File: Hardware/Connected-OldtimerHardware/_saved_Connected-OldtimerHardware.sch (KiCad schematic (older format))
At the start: 20 parts, among them J1 CAN_Bus_Connector, J2 MainConnector, J3 NextionConnector, Q1 2N3906, U1 ParticleElectron, U2 TSR_2-2450, U3 CANTranceiverModule, U4 AdafruitFRAM, U5 AdafruitUltimateGPS, U6 MotionSensor, U7 SFH618A-2

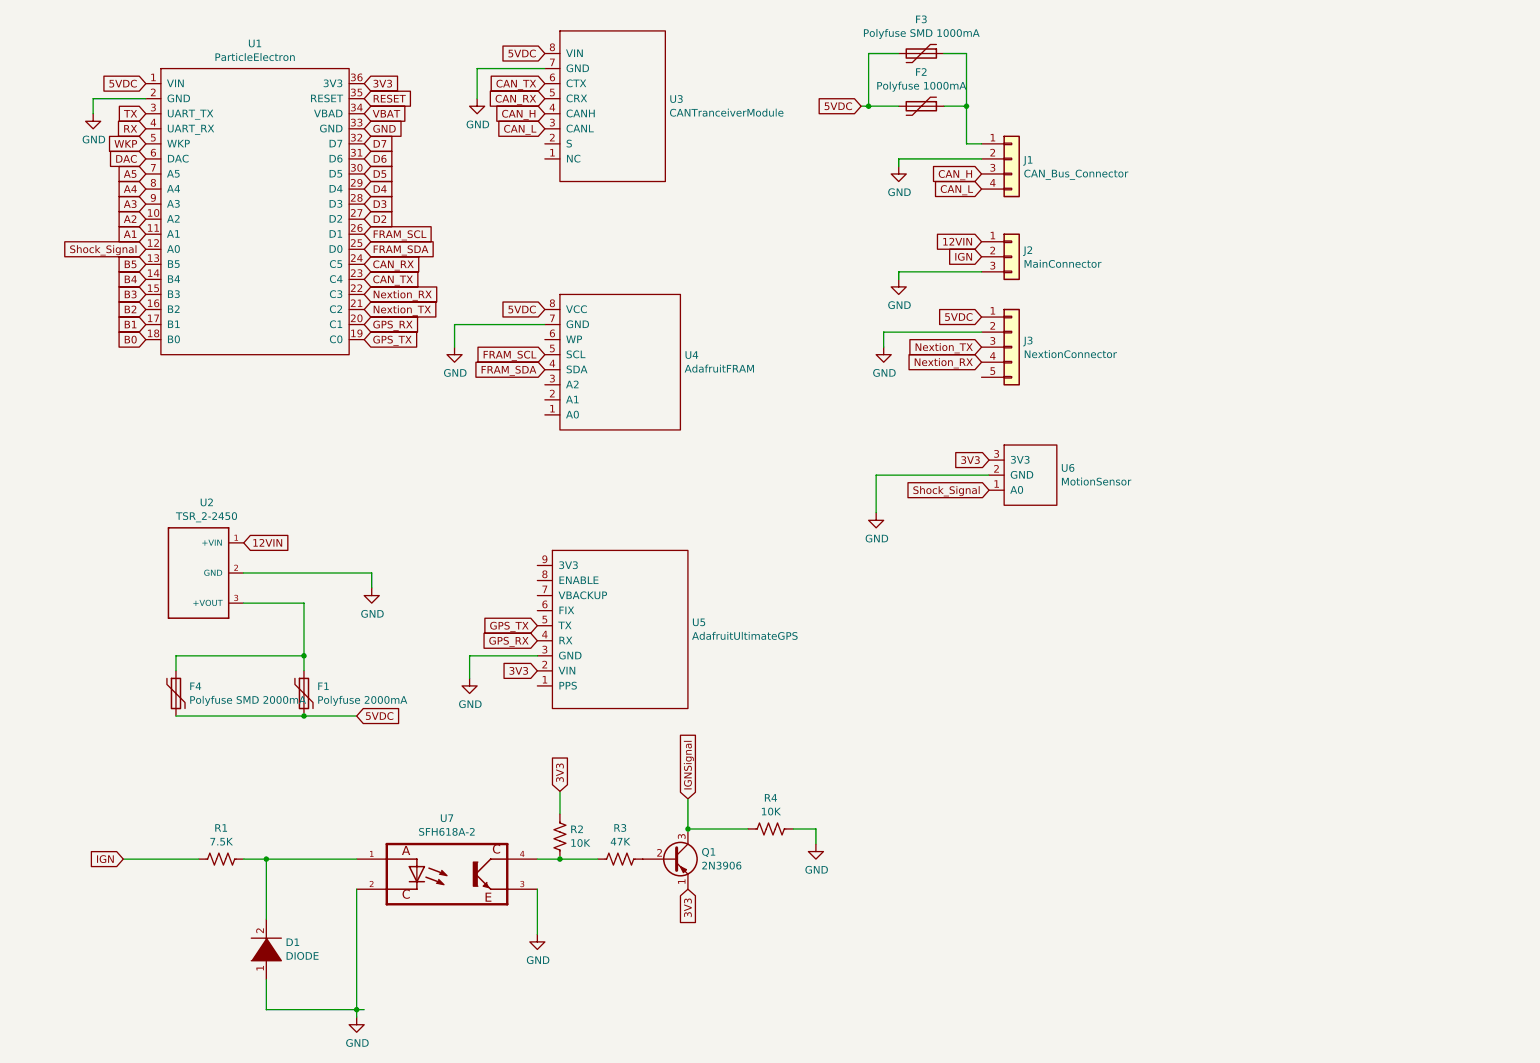
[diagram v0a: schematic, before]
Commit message: layout v1
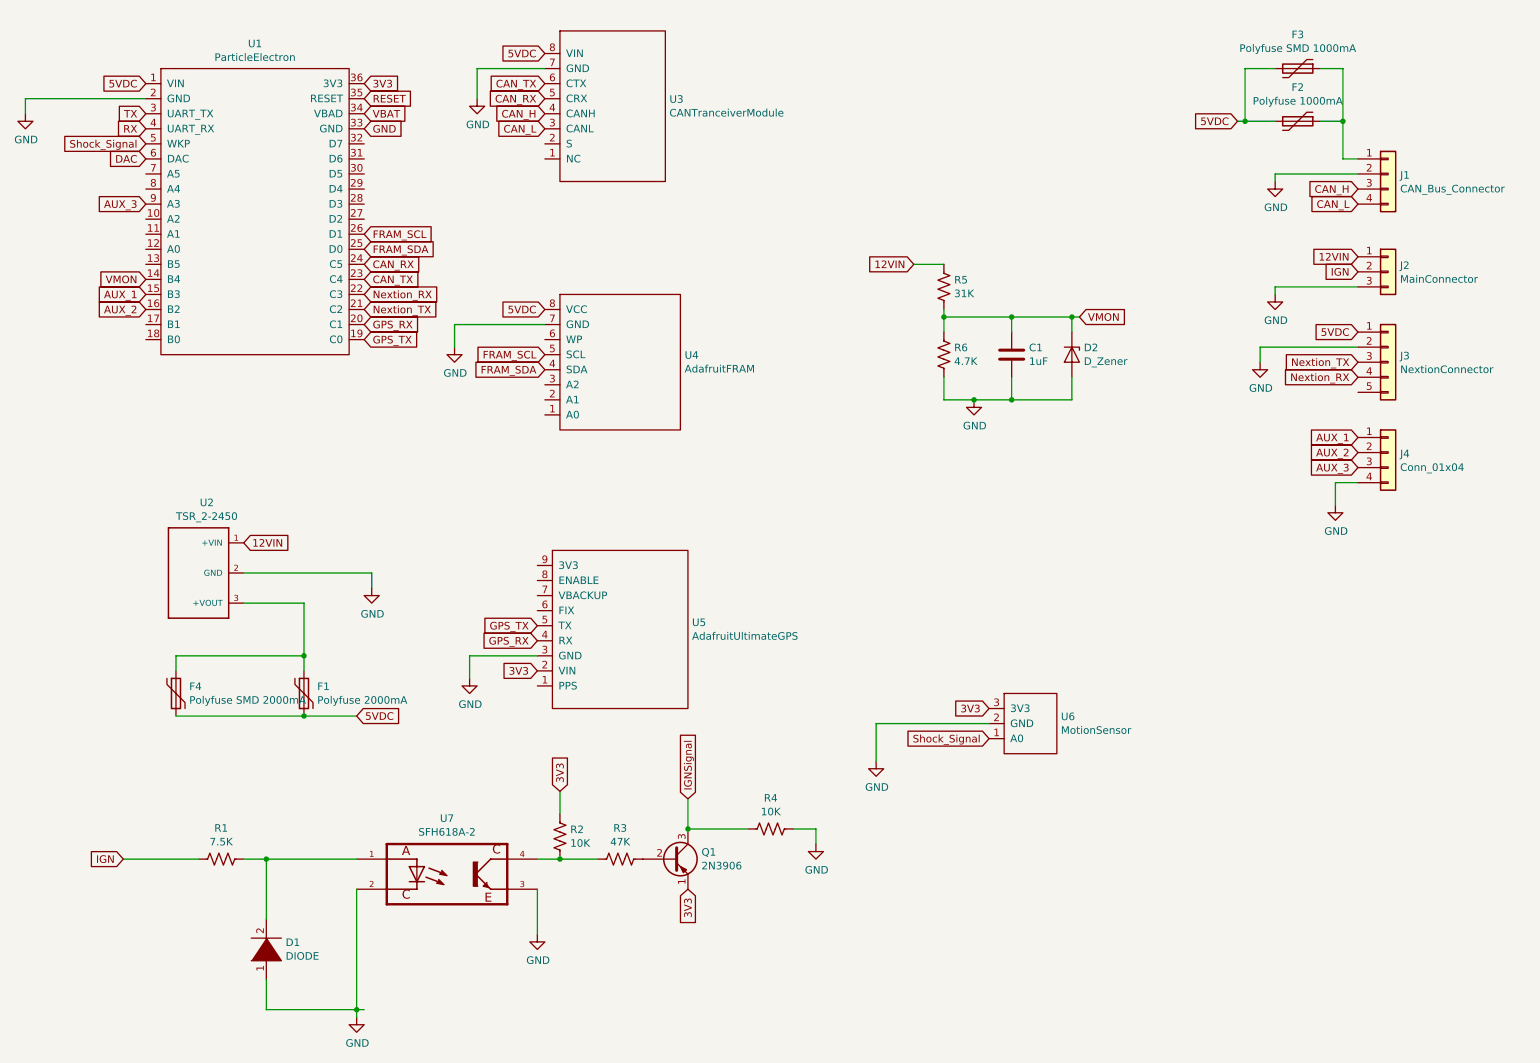
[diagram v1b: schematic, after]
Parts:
- added C1: 1uF, Capacitor_THT:C_Disc_D4.7mm_W2.5mm_P5.00mm, symbol Device:C
- added D2: D_Zener, Diode_THT:D_A-405_P7.62mm_Horizontal, symbol Device:D_Zener
- added J4: Conn_01x04, Connector_JST:JST_XH_B04B-XH-A_1x04_P2.50mm_Vertical, symbol Connector_Generic:Conn_01x04
- added R5: 31K, Resistor_THT:R_Axial_DIN0207_L6.3mm_D2.5mm_P10.16mm_Horizontal, symbol Device:R_US
- added R6: 4.7K, Resistor_THT:R_Axial_DIN0207_L6.3mm_D2.5mm_P10.16mm_Horizontal, symbol Device:R_US
- J1: footprint Connector_JST:JST_EH_B04B-EH-A_1x04_P2.50mm_Vertical -> Connector_JST:JST_XH_B04B-XH-A_1x04_P2.50mm_Vertical
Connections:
- net WKP is gone; now on net Shock_Signal: U1.5 (WKP)
- net 12VIN: now also R5.1
- net GND: now also C1.2, D2.2 (A), J4.4 (Pin_4), R6.2
- net Shock_Signal: no longer U1.12 (A0)
- net A1: no longer names the net of U1.11 (A1)
- net A2: no longer names the net of U1.10 (A2)
- net A3 renamed AUX_3
- net AUX_3: now also J4.3 (Pin_3)
- net A4: no longer names the net of U1.8 (A4)
- net A5: no longer names the net of U1.7 (A5)
- net B0: no longer names the net of U1.18 (B0)
- net B1: no longer names the net of U1.17 (B1)
- net B2 renamed AUX_2
- net AUX_2: now also J4.2 (Pin_2)
- net B3 renamed AUX_1
- net AUX_1: now also J4.1 (Pin_1)
- net B4 renamed VMON
- net VMON: now also C1.1, D2.1 (K), R5.2, R6.1
- net B5: no longer names the net of U1.13 (B5)
- net D2: no longer names the net of U1.27 (D2)
- net D3: no longer names the net of U1.28 (D3)
- net D4: no longer names the net of U1.29 (D4)
- net D5: no longer names the net of U1.30 (D5)
- net D6: no longer names the net of U1.31 (D6)
- net D7: no longer names the net of U1.32 (D7)
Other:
- moved on the sheet: F2, F3, J1, J2, J3, U6
